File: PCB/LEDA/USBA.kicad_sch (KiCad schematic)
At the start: 24 parts, among them J1 USB_A, J2 Conn_01x03, U1 ICS43434_MEMS_Mic, U2 ESP32-S3-MINI-1, U5 MD8942

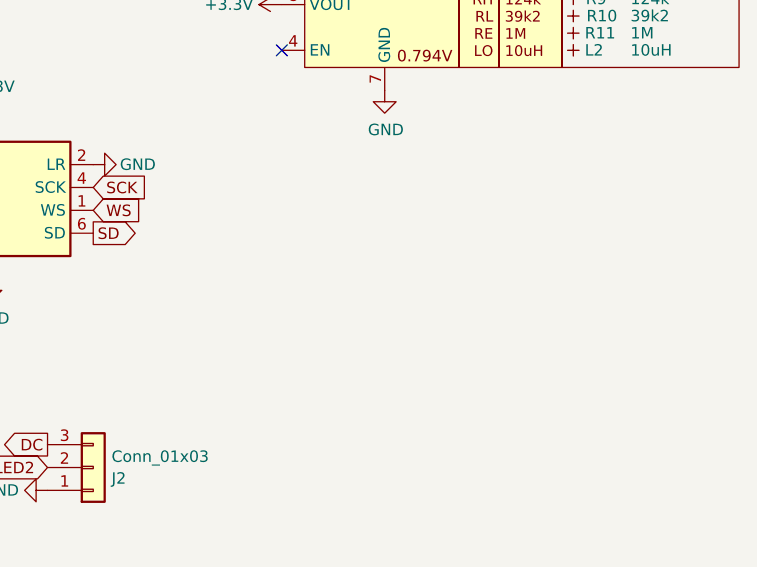
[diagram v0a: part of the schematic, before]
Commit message: Rework
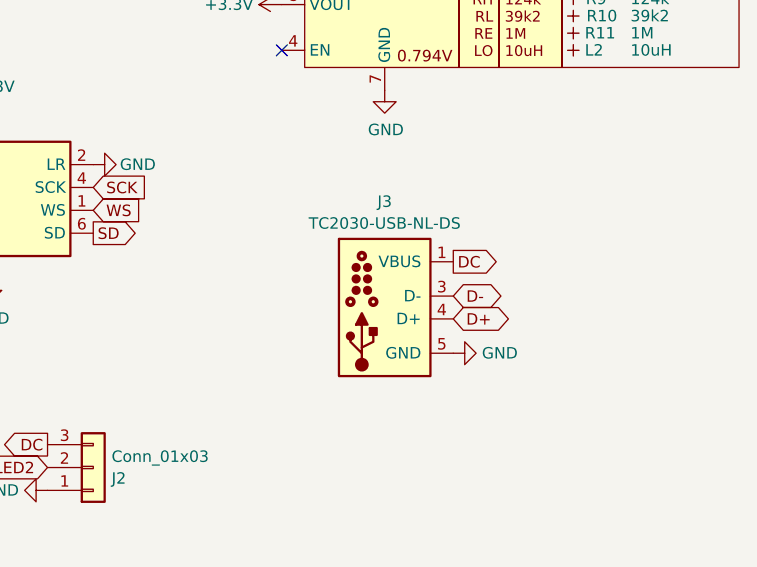
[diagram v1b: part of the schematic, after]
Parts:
- added J3: TC2030-USB-NL-DS, RevK:Tag-Connect_TC2030-IDC-NL_2x03_P1.27mm_Vertical, symbol RevK:TC2030-USB-NL
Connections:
- net D+: now also J3.4 (D+)
- net D-: now also J3.3 (D-)
- net DC: now also J3.1 (VBUS), J3.2 (VBUS)
- net GND: now also J3.5 (GND), J3.6 (GND)
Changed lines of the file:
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@@
+		)
+	)
+	(global_label "D+"
+		(shape bidirectional)
+		(at 241.3 80.645 0)
+		(fields_autoplaced yes)
+		(effects
+			(font
+				(size 1.27 1.27)
+			)
+			(justify left)
+		)
+		(property "Intersheetrefs" "${INTERSHEET_REFS}"
+			(at 247.4259 80.645 0)
+			(effects
+				(font
+					(size 1.27 1.27)
+				)
+				(justify left)
+				(hide yes)
+			)
 		)
 	)
@@
 		)
 	)
+	(global_label "DC"
+		(shape output)
+		(at 241.3 74.295 0)
+		(fields_autoplaced yes)
+		(effects
+			(font
+				(size 1.27 1.27)
+			)
+			(justify left)
+		)
+		(property "Intersheetrefs" "${INTERSHEET_REFS}"
+			(at 246.171 74.295 0)
+			(effects
+				(font
+					(size 1.27 1.27)
+				)
+				(justify left)
+				(hide yes)
+			)
+		)
+	)
 	(global_label "SD"
 		(shape output)
@@
 		(property "Intersheetrefs" "${INTERSHEET_REFS}"
 			(at 206.2869 68.58 0)
+			(effects
+				(font
+					(size 1.27 1.27)
+				)
+				(justify left)
+				(hide yes)
+			)
+		)
+	)
+	(global_label "D-"
+		(shape bidirectional)
+		(at 241.3 78.105 0)
+		(fields_autoplaced yes)
+		(effects
+			(font
+				(size 1.27 1.27)
+			)
+			(justify left)
+		)
+		(property "Intersheetrefs" "${INTERSHEET_REFS}"
+			(at 247.4259 78.105 0)
 			(effects
 				(font
@@
 	)
 	(symbol
+		(lib_id "RevK:TC2030-USB-NL")
+		(at 233.68 79.375 0)
+		(unit 1)
+		(exclude_from_sim no)
+		(in_bom no)
+		(on_board yes)
+		(dnp no)
+		(fields_autoplaced yes)
+		(property "Reference" "J3"
+			(at 233.68 67.6105 0)
+			(effects
+				(font
+					(size 1.27 1.27)
+				)
+			)
+		)
+		(property "Value" "TC2030-USB-NL-DS"
+			(at 233.68 70.0348 0)
+			(effects
+				(font
+					(size 1.27 1.27)
+				)
+			)
+		)
+		(property "Footprint" "RevK:Tag-Connect_TC2030-IDC-NL_2x03_P1.27mm_Vertical"
+			(at 233.426 88.519 0)
+			(effects
+				(font
+					(size 1.27 1.27)
+				)
+				(hide yes)
+			)
+		)
+		(property "Datasheet" " ~"
+			(at 237.49 80.645 0)
+			(effects
+				(font
+					(size 1.27 1.27)
+				)
+				(hide yes)
+			)
+		)
+		(property "Description" "TC2030-USB-NL"
+			(at 233.68 66.675 0)
+			(effects
+				(font
+					(size 1.27 1.27)
+				)
+				(hide yes)
+			)
+		)
+		(pin "1"
+		)
+		(pin "2"
+		)
+		(pin "3"
+		)
+		(pin "4"
+		)
+		(pin "5"
+		)
+		(pin "6"
+		)
+		(instances
+			(project "USBA"
+				(path "/2d210a96-f81f-42a9-8bf4-1b43c11086f3"
+					(reference "J3")
+					(unit 1)
+				)
+			)
+		)
+	)
+	(symbol
 		(lib_id "power:+3.3V")
 		(at 222.25 45.72 90)
@@
 					(unit 1)
 				)
+			)
+		)
+	)
+	(symbol
+		(lib_id "power:GND")
+		(at 241.3 84.455 90)
+		(unit 1)
+		(exclude_from_sim no)
+		(in_bom yes)
+		(on_board yes)
+		(dnp no)
+		(fields_autoplaced yes)
+		(property "Reference" "#PWR015"
+			(at 247.65 84.455 0)
+			(effects
+				(font
+					(size 1.27 1.27)
+				)
+				(hide yes)
+			)
+		)
+		(property "Value" "GND"
+			(at 244.475 84.455 90)
+			(effects
+				(font
+					(size 1.27 1.27)
+				)
+				(justify right)
+			)
+		)
+		(property "Footprint" ""
+			(at 241.3 84.455 0)
+			(effects
+				(font
+					(size 1.27 1.27)
+				)
+				(hide yes)
+			)
+		)
+		(property "Datasheet" ""
+			(at 241.3 84.455 0)
+			(effects
+				(font
+					(size 1.27 1.27)
+				)
+				(hide yes)
+			)
+		)
+		(property "Description" "Power symbol creates a global label with name \"GND\" , ground"
+			(at 241.3 84.455 0)
+			(effects
+				(font
+					(size 1.27 1.27)
+				)
+				(hide yes)
+			)
+		)
+		(pin "1"
+		)
+		(instances
+			(project "USBA"
+				(path "/2d210a96-f81f-42a9-8bf4-1b43c11086f3"
+					(reference "#PWR015")
+					(unit 1)
+				)
